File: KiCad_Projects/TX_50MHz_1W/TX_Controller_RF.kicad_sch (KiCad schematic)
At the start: 37 parts, among them J1 AIL Stick, J10 I2C Exp / OLED, J11 ANT, J2 ELE Stick, J3 THR Stick, J4 RUD Stick, J5 AUX6, J6 AUX5, J7 AUX7, Q1 RD01MUS2 (1W PA), U1 ESP32-S3-WROOM-1-N16R8, U2 Si5351A-B-GT, U3 BGS12SN6E6327XTSA1 (T/R SW), U4 SPF5043Z (LNA), U5 LT5560 (Mixer), U6 ADS1115IDGSR (0x48), U7 ADS1115IDGSR (0x49), U8 SH1106 1.3in OLED, Y1 26.000MHz

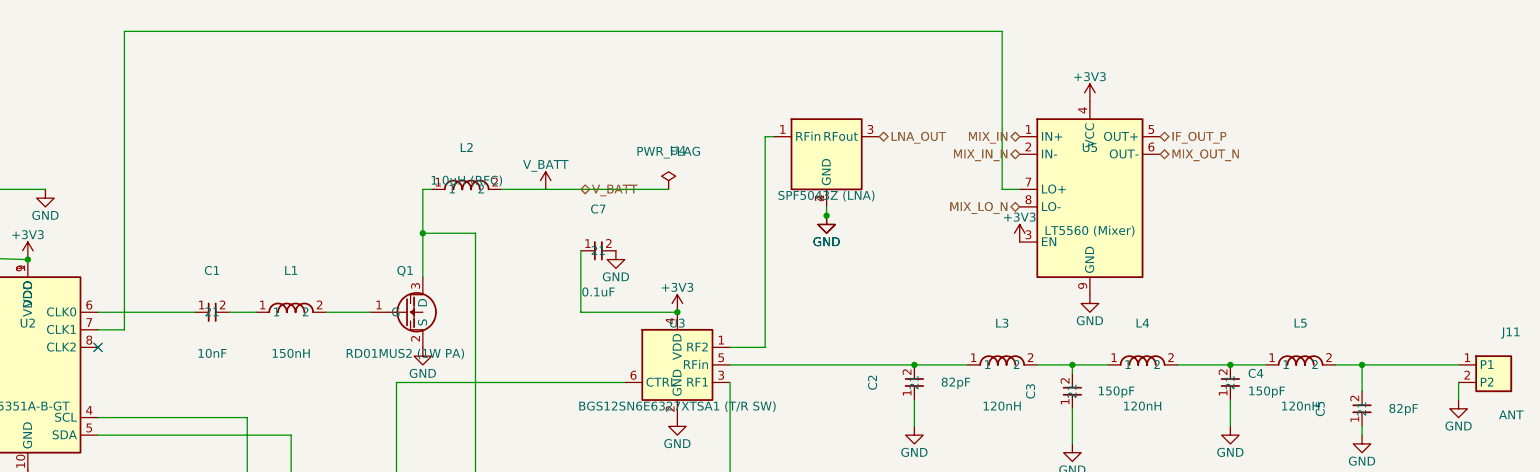
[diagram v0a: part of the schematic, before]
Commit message: udated scheamatic
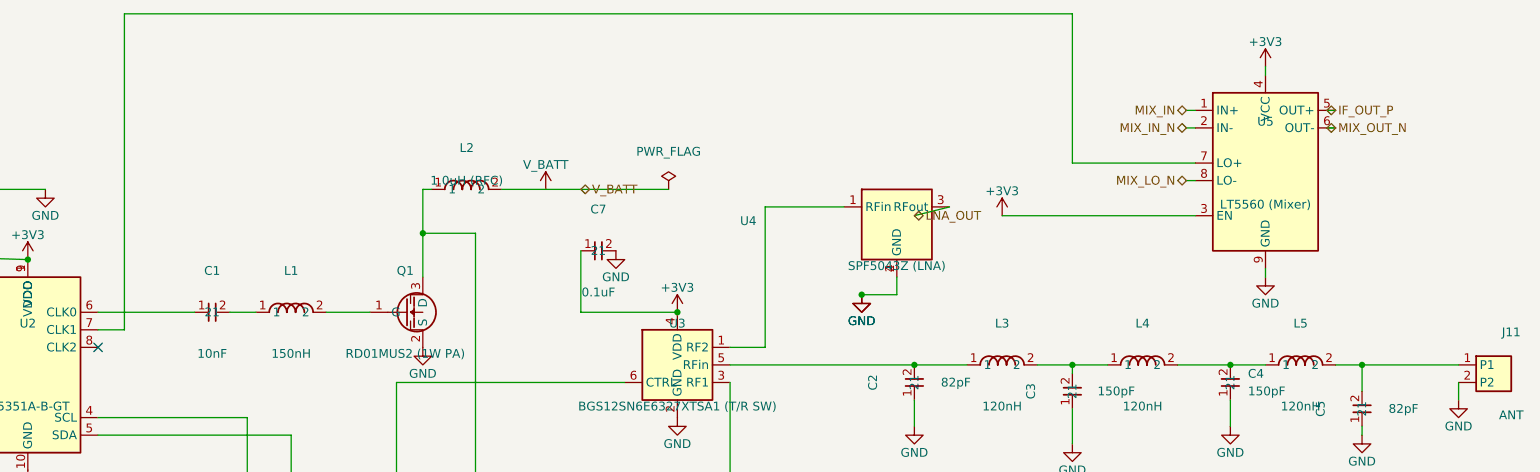
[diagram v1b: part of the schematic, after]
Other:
- moved on the sheet: U4, U5
